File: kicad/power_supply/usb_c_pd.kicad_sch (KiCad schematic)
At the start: 39 parts, among them J201 Conn_01x04_Socket, J202 12401826E412A, J203 Conn_01x03_Socket, SW201 SW_SPST, U201 USBLC6-2SC6, U202 STUSB4500QTR

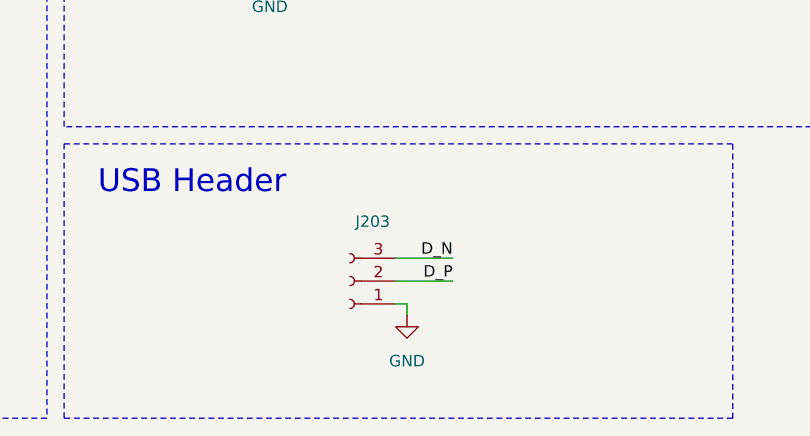
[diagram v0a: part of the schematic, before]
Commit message: psu buck-boost schematic capture
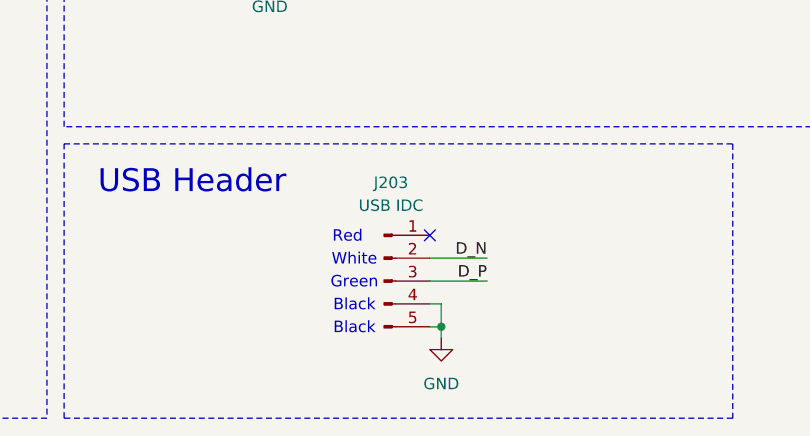
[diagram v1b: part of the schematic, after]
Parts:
- removed J203: Conn_01x03_Socket, symbol Connector:Conn_01x03_Socket
- added J203: USB IDC, symbol Connector:Conn_01x05_Pin
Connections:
- net D_N: now also J203.2 (Pin_2)
- net D_P: now also J203.3 (Pin_3)
- net GND: now also J203.4 (Pin_4), J203.5 (Pin_5)
- no-connect marks 12 -> 13
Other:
- note added: "Black"
- note added: "Green"
- note added: "Red"
- note added: "White"
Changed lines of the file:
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@@
 	)
 	(junction
+		(at 140.97 184.15)
+		(diameter 0)
+		(color 0 0 0 0)
+	)
+	(junction
 		(at 227.33 43.18)
 		(diameter 0)
@@
 	)
 	(no_connect
+		(at 139.7 173.99)
+	)
+	(no_connect
 		(at 137.16 130.81)
 	)
@@
 	(wire
 		(pts
-			(xy 142.24 179.07) (xy 135.89 179.07)
+			(xy 146.05 179.07) (xy 139.7 179.07)
 		)
 		(stroke
@@
 	(wire
 		(pts
+			(xy 140.97 181.61) (xy 140.97 184.15)
+		)
+		(stroke
+			(width 0)
+			(type default)
+		)
+	)
+	(wire
+		(pts
 			(xy 90.17 35.56) (xy 85.09 35.56)
 		)
@@
 	(wire
 		(pts
-			(xy 142.24 176.53) (xy 135.89 176.53)
+			(xy 146.05 176.53) (xy 139.7 176.53)
 		)
 		(stroke
@@
 	(wire
 		(pts
+			(xy 139.7 181.61) (xy 140.97 181.61)
+		)
+		(stroke
+			(width 0)
+			(type default)
+		)
+	)
+	(wire
+		(pts
 			(xy 22.86 39.37) (xy 22.86 40.64)
 		)
@@
 	(wire
 		(pts
-			(xy 135.89 181.61) (xy 137.16 181.61)
+			(xy 139.7 184.15) (xy 140.97 184.15)
 		)
 		(stroke
@@
 	(wire
 		(pts
-			(xy 137.16 181.61) (xy 137.16 182.88)
+			(xy 140.97 184.15) (xy 140.97 185.42)
 		)
 		(stroke
@@
 		)
 	)
+	(text "Black"
+		(exclude_from_sim no)
+		(at 131.318 184.404 0)
+		(effects
+			(font
+				(size 1.27 1.27)
+			)
+		)
+	)
+	(text "Green"
+		(exclude_from_sim no)
+		(at 131.318 179.324 0)
+		(effects
+			(font
+				(size 1.27 1.27)
+			)
+		)
+	)
 	(text "Reset Switch"
 		(exclude_from_sim no)
@@
 		)
 	)
+	(text "Red"
+		(exclude_from_sim no)
+		(at 130.556 174.244 0)
+		(effects
+			(font
+				(size 1.27 1.27)
+			)
+		)
+	)
 	(text "USB Header"
 		(exclude_from_sim no)
@@
 		)
 	)
+	(text "Black"
+		(exclude_from_sim no)
+		(at 131.318 181.864 0)
+		(effects
+			(font
+				(size 1.27 1.27)
+			)
+		)
+	)
+	(text "White"
+		(exclude_from_sim no)
+		(at 131.318 176.784 0)
+		(effects
+			(font
+				(size 1.27 1.27)
+			)
+		)
+	)
 	(text "ADDR0 | ADDR1 | Address\n  0    |   0    | 0x28*\n  0    |   1    | 0x29\n  1    |   0    | 0x2A\n  1    |   1    | 0x2B\n\n*: Default\n0: Jumper closed\n1: Jumper open"
 		(exclude_from_sim no)
@@
 	)
 	(label "D_P"
-		(at 142.24 179.07 180)
+		(at 146.05 179.07 180)
 		(fields_autoplaced yes)
 		(effects
@@
 	)
 	(label "D_N"
-		(at 142.24 176.53 180)
+		(at 146.05 176.53 180)
 		(fields_autoplaced yes)
 		(effects
@@
 	)
 	(symbol
+		(lib_id "Connector:Conn_01x05_Pin")
+		(at 134.62 179.07 0)
+		(unit 1)
+		(exclude_from_sim no)
+		(in_bom yes)
+		(on_board yes)
+		(dnp no)
+		(property "Reference" "J203"
+			(at 135.382 168.148 0)
+			(effects
+				(font
+					(size 1.27 1.27)
+				)
+			)
+		)
+		(property "Value" "USB IDC"
+			(at 135.382 170.688 0)
+			(effects
+				(font
+					(size 1.27 1.27)
+				)
+			)
+		)
+		(property "Footprint" ""
+			(at 134.62 179.07 0)
+			(effects
+				(font
+					(size 1.27 1.27)
+				)
+				(hide yes)
+			)
+		)
+		(property "Datasheet" "~"
+			(at 134.62 179.07 0)
+			(effects
+				(font
+					(size 1.27 1.27)
+				)
+				(hide yes)
+			)
+		)
+		(property "Description" "Generic connector, single row, 01x05, script generated"
+			(at 134.62 179.07 0)
+			(effects
+				(font
+					(size 1.27 1.27)
+				)
+				(hide yes)
+			)
+		)
+		(pin "3"
+		)
+		(pin "1"
+		)
+		(pin "4"
+		)
+		(pin "2"
+		)
+		(pin "5"
+		)
+		(instances
+			(project ""
+				(path "/6a7d9dc9-f78f-470f-911b-b95256023173/4a384965-6a35-4bf6-849e-cb865e62d5b4"
+					(reference "J203")
+					(unit 1)
+				)
+			)
+		)
+	)
+	(symbol
 		(lib_id "Device:R_Small_US")
 		(at 260.35 57.15 0)
@@
 	(symbol
 		(lib_id "power:GND")
-		(at 137.16 182.88 0)
+		(at 140.97 185.42 0)
 		(unit 1)
 		(exclude_from_sim no)
@@
 		(fields_autoplaced yes)
 		(property "Reference" "#PWR0206"
-			(at 137.16 189.23 0)
+			(at 140.97 191.77 0)
 			(effects
 				(font
@@
 		)
 		(property "Value" "GND"
-			(at 137.16 187.96 0)
+			(at 140.97 190.5 0)
 			(effects
 				(font
@@
 		)
 		(property "Footprint" ""
-			(at 137.16 182.88 0)
+			(at 140.97 185.42 0)
 			(effects
 				(font
@@
 		)
 		(property "Datasheet" ""
-			(at 137.16 182.88 0)
+			(at 140.97 185.42 0)
 			(effects
 				(font
@@
 		)
 		(property "Description" "Power symbol creates a global label with name \"GND\" , ground"
-			(at 137.16 182.88 0)
+			(at 140.97 185.42 0)
 			(effects
 				(font
@@
 					(unit 1)
 				)
-			)
-		)
-	)
-	(symbol
-		(lib_id "Connector:Conn_01x03_Socket")
-		(at 130.81 179.07 180)
-		(unit 1)
-		(exclude_from_sim no)
-		(in_bom yes)
-		(on_board yes)
-		(dnp no)
-		(property "Reference" "J203"
-			(at 133.35 172.466 0)
-			(effects
-				(font
-					(size 1.27 1.27)
-				)
-			)
-		)
-		(property "Value" "Conn_01x03_Socket"
-			(at 131.445 173.99 0)
-			(effects
-				(font
-					(size 1.27 1.27)
-				)
-				(hide yes)
-			)
-		)
-		(property "Footprint" ""
-			(at 130.81 179.07 0)
-			(effects
-				(font
-					(size 1.27 1.27)
-				)
-				(hide yes)
-			)
-		)
-		(property "Datasheet" "~"
-			(at 130.81 179.07 0)
-			(effects
-				(font
-					(size 1.27 1.27)
-				)
-				(hide yes)
-			)
-		)
-		(property "Description" "Generic connector, single row, 01x03, script generated"
-			(at 130.81 179.07 0)
-			(effects
-				(font
-					(size 1.27 1.27)
-				)
-				(hide yes)
-			)
-		)
-		(pin "3"
-		)
-		(pin "1"
-		)
-		(pin "2"
-		)
-		(instances
-			(project ""
-				(path "/6a7d9dc9-f78f-470f-911b-b95256023173/4a384965-6a35-4bf6-849e-cb865e62d5b4"
-					(reference "J203")
-					(unit 1)
-				)
